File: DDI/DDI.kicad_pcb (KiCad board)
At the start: 2 copper layers, 54 parts, among them J1 Conn_01x06_Socket, J2 Conn_02x04_Top_Bottom, Q1 Q_NMOS_GDS, SW1 SW_Push, SW10 SW_Push, SW11 SW_Push, SW12 SW_Push, SW13 SW_Push, SW14 SW_Push, SW15 SW_Push, SW16 SW_Push, SW17 SW_Push, SW18 SW_Push, SW19 SW_Push, SW2 SW_Push, SW20 SW_Push, SW3 SW_Push, SW4 SW_Push, SW5 SW_Push, SW6 SW_Push, SW7 SW_Push, SW8 SW_Push, SW9 SW_Push, U1 ADS1015IDGS, U2 MCP23017_SP, U3 MCP23017_SP

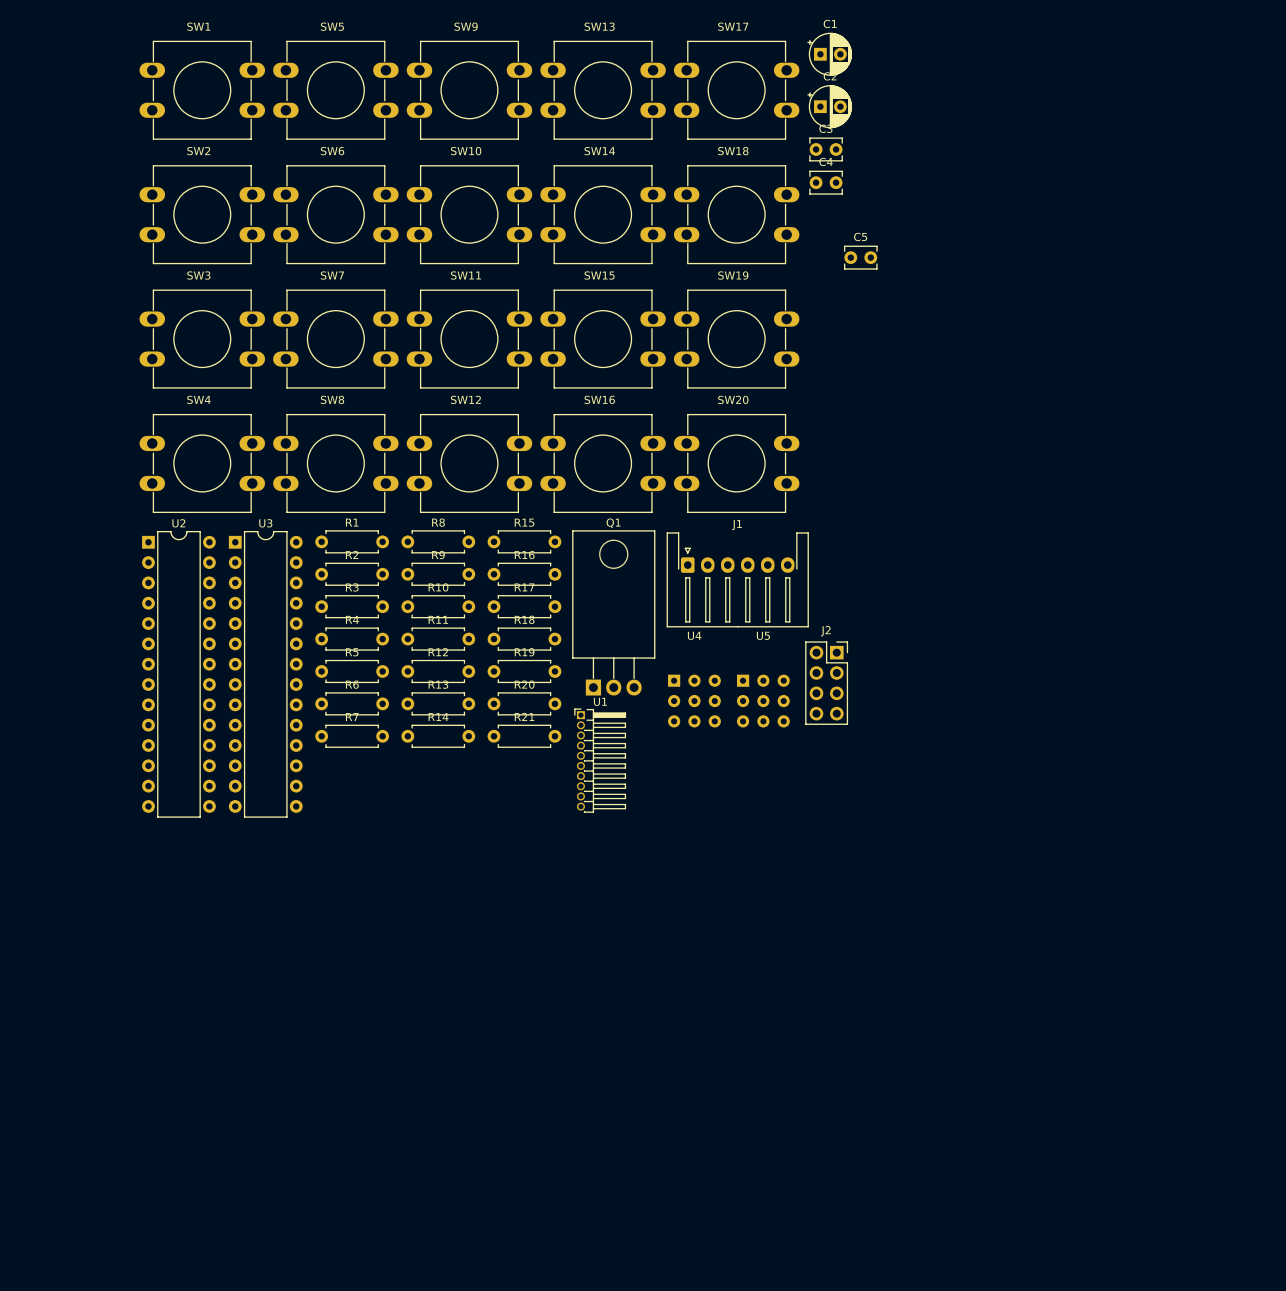
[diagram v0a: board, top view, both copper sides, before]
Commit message: DDIを変更
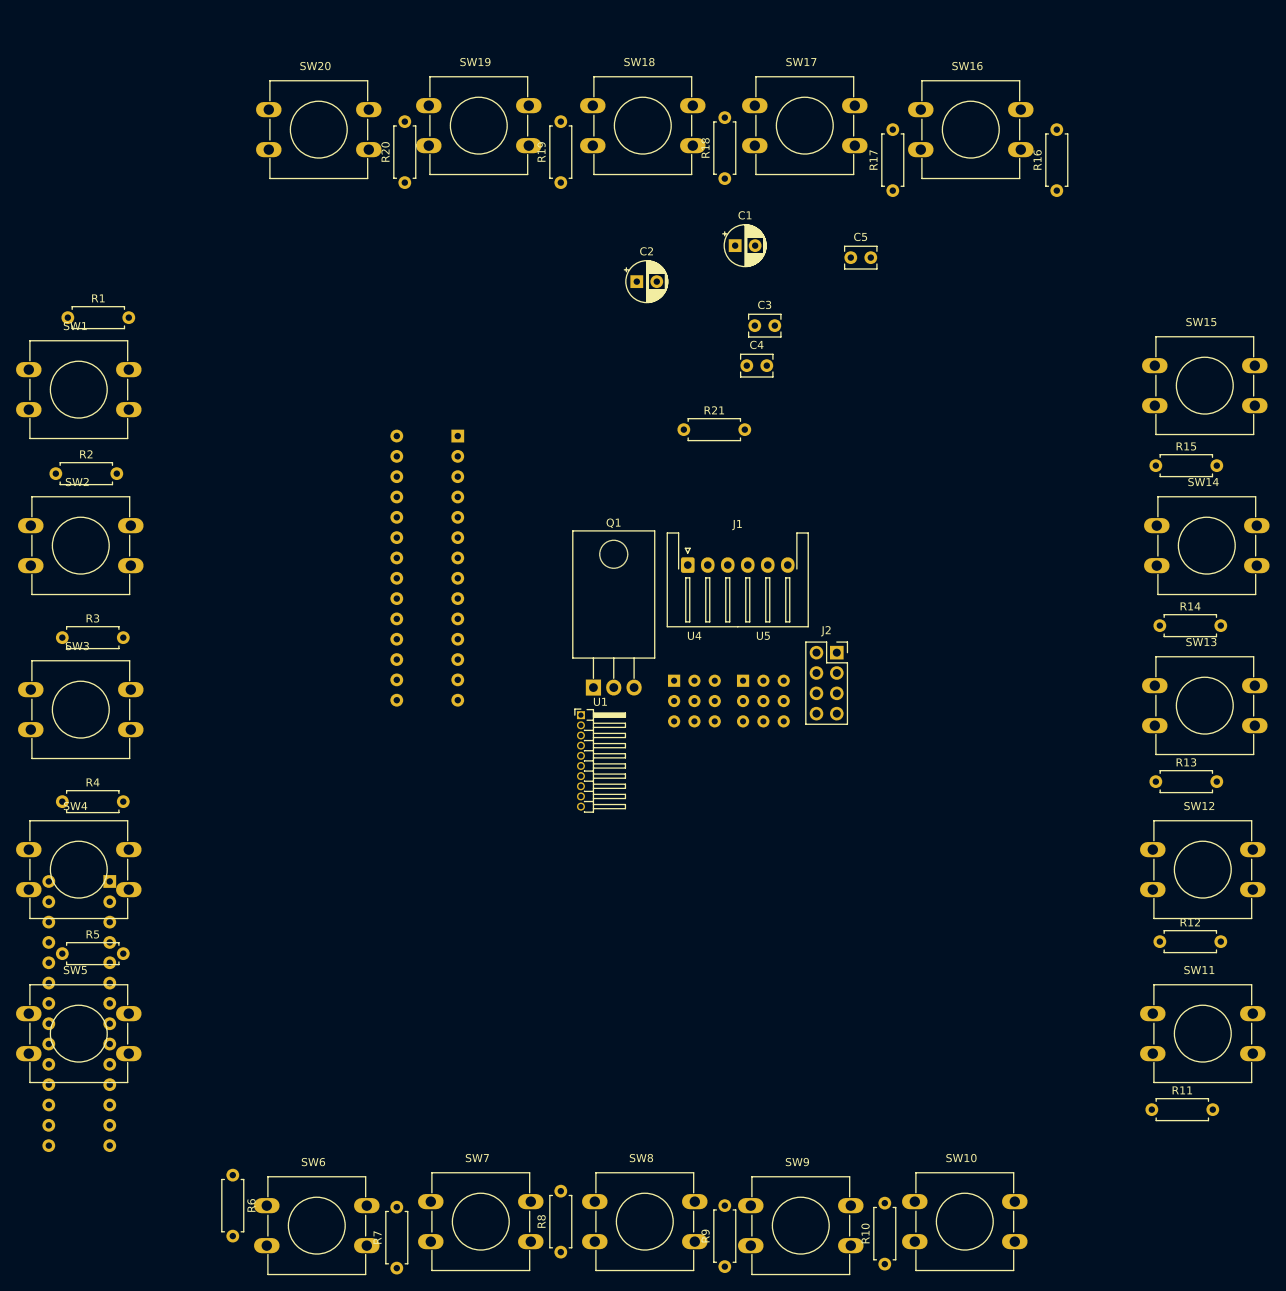
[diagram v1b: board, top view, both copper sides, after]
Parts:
- U2, U3: moved to B.Cu
- moved SW9 147.8 mm to (130.2, 176.5)
- moved SW10 140.3 mm to (150.8, 176.0)
- moved SW6 126.4 mm to (69.8, 176.5)
- moved SW11 126.3 mm to (180.5, 152.5)
- moved SW5 122.2 mm to (40.0, 152.5)
- moved SW7 111.8 mm to (90.2, 176.0)
- moved R11 110.0 mm to (180.4, 164.5)
- moved SW13 107.6 mm to (180.8, 111.5)
- moved SW12 104.8 mm to (180.5, 132.0)
- moved SW8 102.3 mm to (110.8, 176.0)
- moved R10 101.5 mm to (147.0, 183.8), turned to 90 degrees
- moved R12 99.9 mm to (181.4, 143.5)
- moved R9 95.2 mm to (127.0, 184.1), turned to 90 degrees
- moved R14 95.0 mm to (181.4, 104.0)
- moved R13 94.0 mm to (180.9, 123.5)
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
